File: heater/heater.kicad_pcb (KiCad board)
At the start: 2 copper layers, 100 x 100 mm, 0 parts

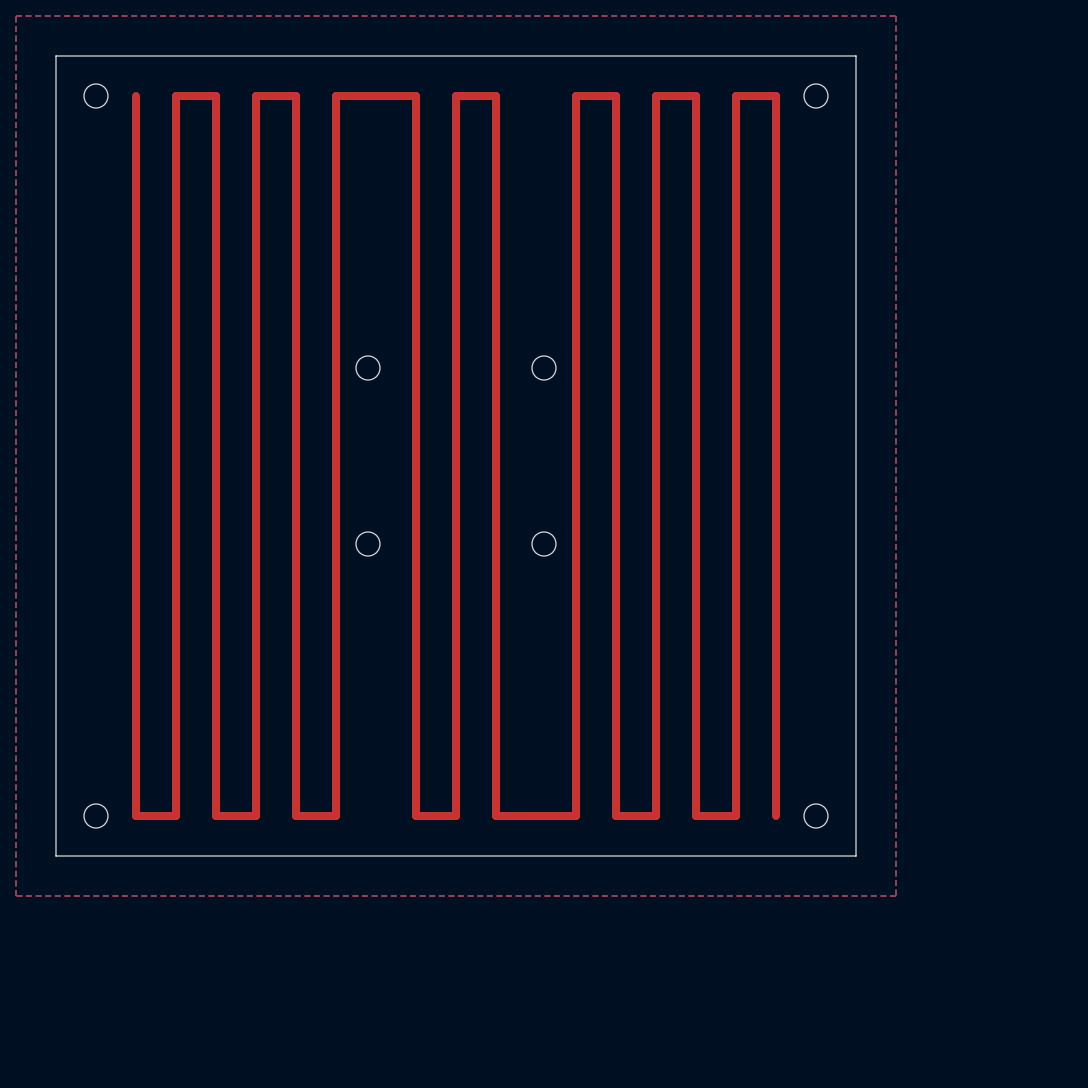
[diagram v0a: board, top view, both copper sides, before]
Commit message: 6 ohm nominal version of heater board
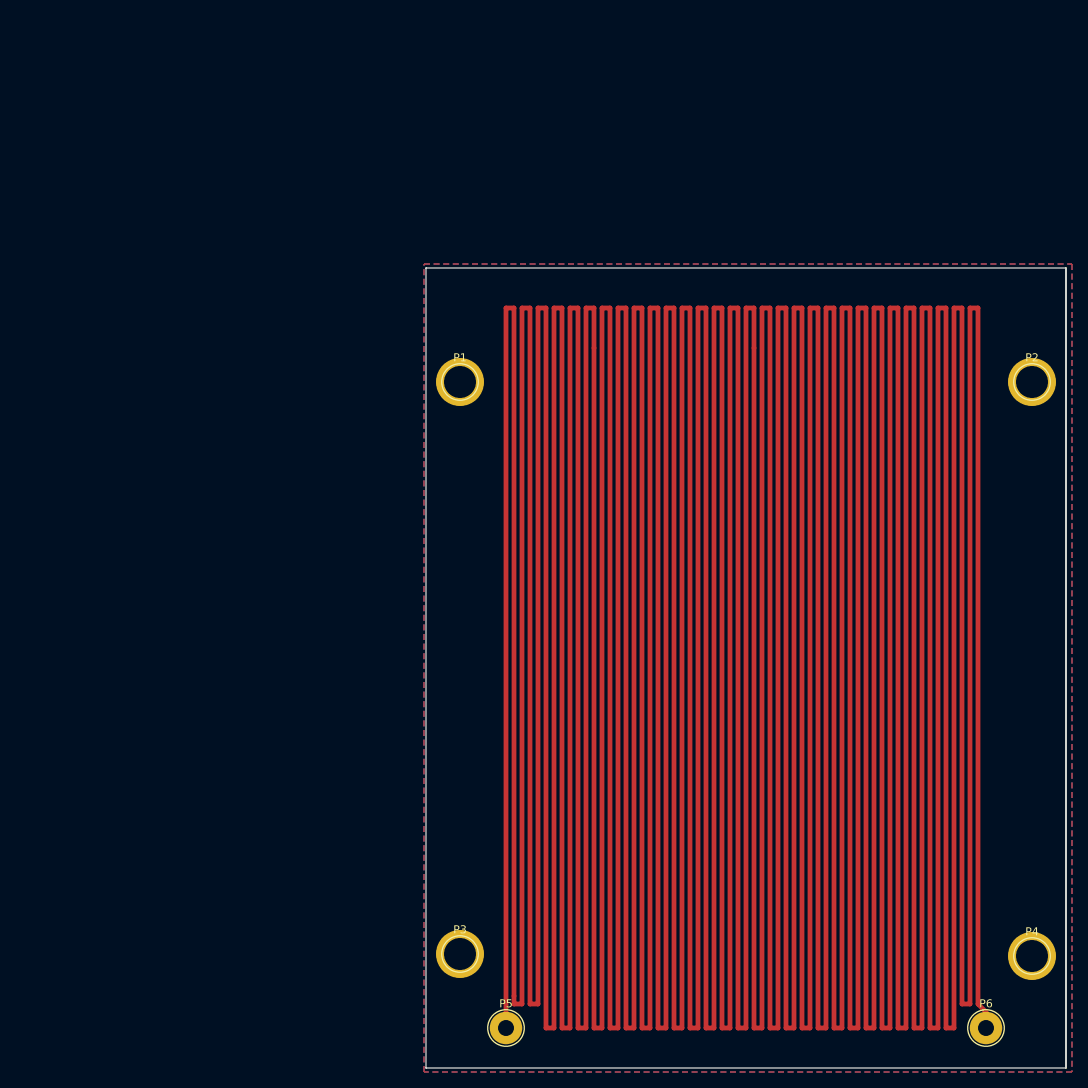
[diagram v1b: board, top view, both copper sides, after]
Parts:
- added P1: CONN_01X01, Connect:1pin, F.Cu at (75.5, 65.8)
- added P2: CONN_01X01, Connect:1pin, F.Cu at (147.0, 65.8)
- added P3: CONN_01X01, Connect:1pin, F.Cu at (75.5, 137.2)
- added P4: CONN_01X01, Connect:1pin, F.Cu at (147.0, 137.5)
- added P5: CONN_01X01, Connect:1pin, F.Cu at (81.2, 146.5)
- added P6: CONN_01X01, Connect:1pin, F.Cu at (141.2, 146.5)
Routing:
- net Net-(P5-Pad1): track 0.00 -> 5441.4 mm
- net (no net): track 1430.0 -> 0.00 mm
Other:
- board size 100 x 100 mm -> 80 x 100 mm
